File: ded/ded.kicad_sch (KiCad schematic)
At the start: 2 parts, among them J1 USB_C_Receptacle_PowerOnly_6P, J2 USB_C_Receptacle_PowerOnly_6P

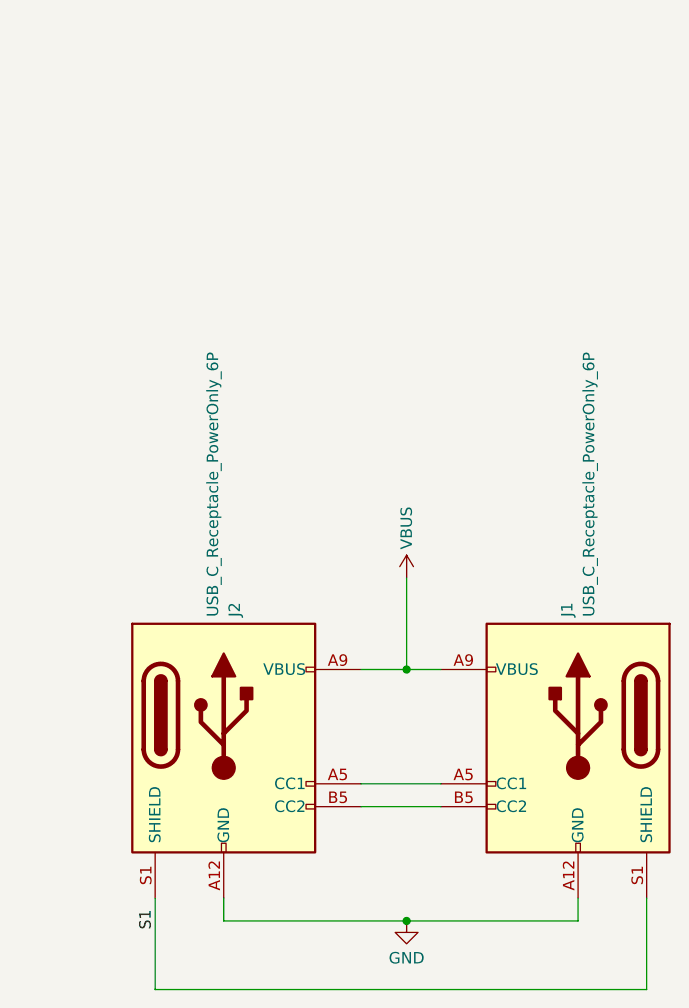
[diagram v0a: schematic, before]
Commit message: candidate designs for ded and deh couplers
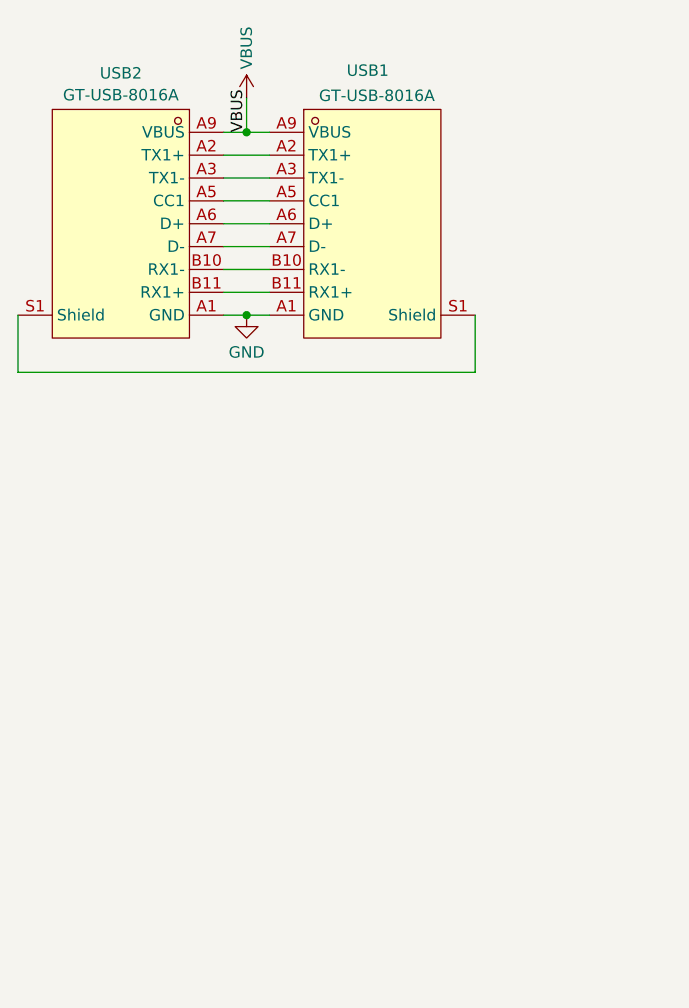
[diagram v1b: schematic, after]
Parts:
- removed J1, J2: USB_C_Receptacle_PowerOnly_6P, ded:TYPE-C-SMD_TYPE-C-6P_5, symbol Connector:USB_C_Receptacle_PowerOnly_6P
- added USB1, USB2: GT-USB-8016A, ded:USB-TYPE-C-SMD_GT-USB-8016A, symbol ded:GT-USB-8016A
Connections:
- net GND: now also USB1.A1 (GND), USB2.A1 (GND)
- net VBUS: now also USB1.A9 (VBUS), USB2.A9 (VBUS)
- new net: USB1.A2 (TX1+), USB2.A2 (TX1+)
- new net: USB1.A3 (TX1-), USB2.A3 (TX1-)
- new net: USB1.A5 (CC1), USB2.A5 (CC1)
- new net: USB1.A6 (D+), USB2.A6 (D+)
- new net: USB1.A7 (D-), USB2.A7 (D-)
- new net: USB1.B10 (RX1-), USB2.B10 (RX1-)
- new net: USB1.B11 (RX1+), USB2.B11 (RX1+)
- new net: USB1.S1 (Shield), USB2.S1 (Shield)
